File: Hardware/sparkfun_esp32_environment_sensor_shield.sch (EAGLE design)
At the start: 53 parts, among them J1 WEATHER_METER-WIND, J2 WEATHER_METER-RAIN, U1 BME280, U2 CCS811, U3 APDS-9301, U4 TVS Diode

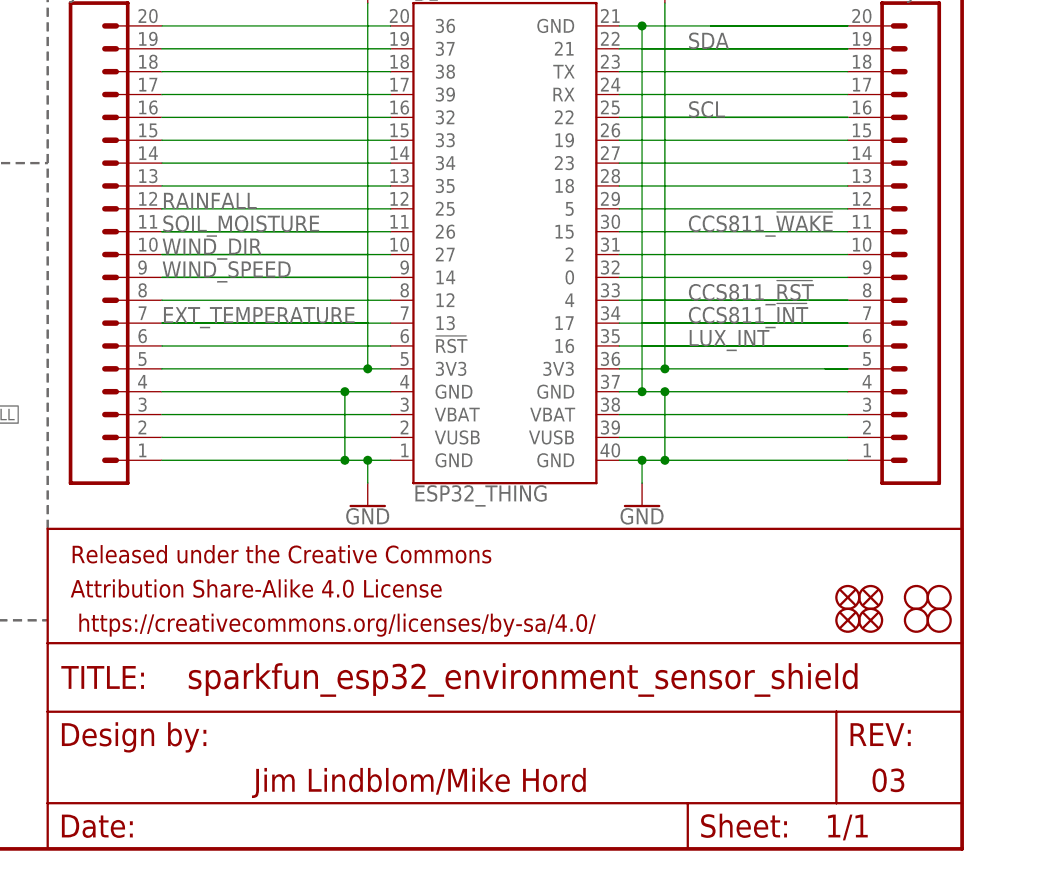
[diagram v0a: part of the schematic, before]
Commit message: Changes from review
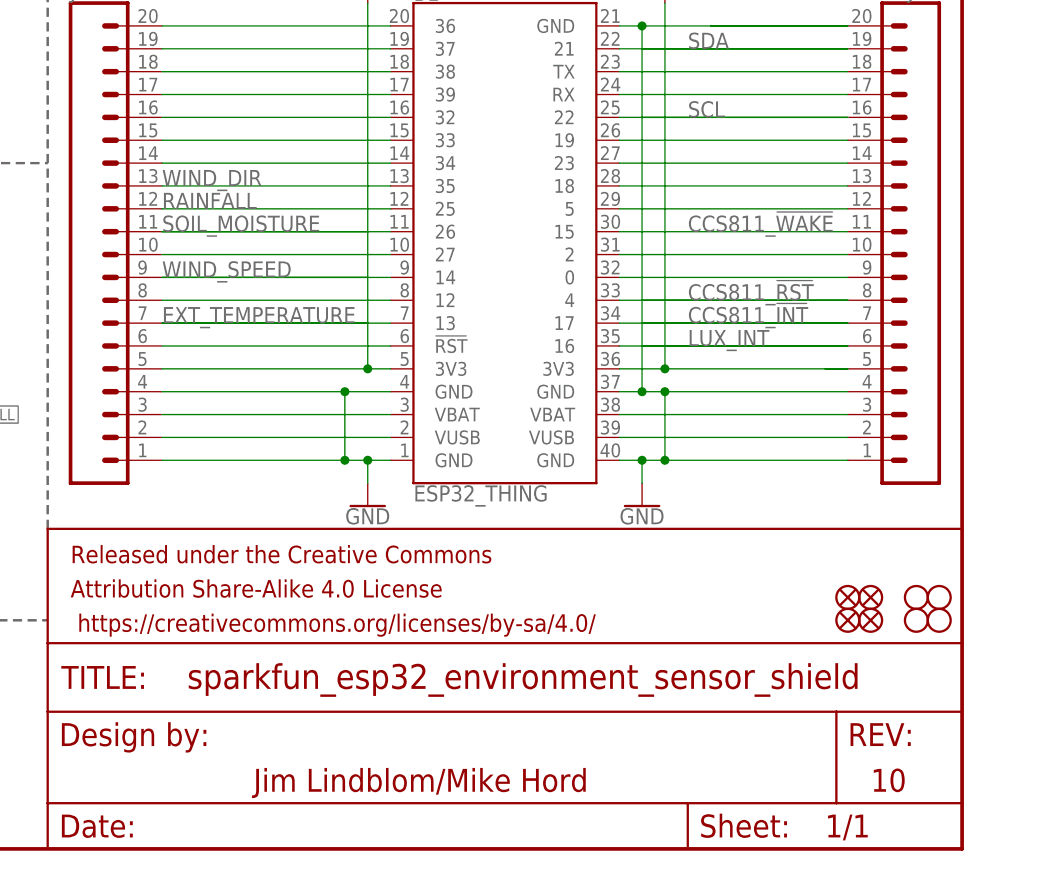
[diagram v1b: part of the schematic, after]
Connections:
- removed net N$10: B1.35, J4.13
- new net N$9: B1.27, J4.10
- net WIND_DIR: now also B1.35, J4.13; no longer B1.27, J4.10
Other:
- note added: "10"
- note removed: "03"
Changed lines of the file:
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@@
 to 4.7k pull-up
 resistors.</text>
-<text x="238.76" y="7.62" size="2.54" layer="94" align="center-left">03</text>
+<text x="238.76" y="7.62" size="2.54" layer="94" align="center-left">10</text>
 <text x="170.18" y="7.62" size="2.54" layer="94" align="center-left">Jim Lindblom/Mike Hord</text>
 <text x="119.38" y="20.32" size="1.27" layer="97" align="top-left">3-Pin temperature
@@
 </segment>
 <segment>
-<pinref part="B1" gate="G$1" pin="27"/>
-<wire x1="160.02" y1="66.04" x2="182.88" y2="66.04" width="0.1524" layer="91"/>
-<pinref part="J4" gate="G$1" pin="10"/>
-<wire x1="160.02" y1="66.04" x2="185.42" y2="66.04" width="0.1524" layer="91"/>
-<label x="160.02" y="66.04" size="1.778" layer="95"/>
-</segment>
-<segment>
 <wire x1="73.66" y1="58.42" x2="71.12" y2="58.42" width="0.1524" layer="91"/>
 <pinref part="U4" gate="U1" pin="IO4"/>
 <wire x1="73.66" y1="55.88" x2="73.66" y2="58.42" width="0.1524" layer="91"/>
 <label x="71.12" y="58.42" size="1.27" layer="95" rot="R180" xref="yes"/>
+</segment>
+<segment>
+<pinref part="B1" gate="G$1" pin="35"/>
+<pinref part="J4" gate="G$1" pin="13"/>
+<wire x1="160.02" y1="73.66" x2="185.42" y2="73.66" width="0.1524" layer="91"/>
+<label x="160.02" y="73.66" size="1.778" layer="95"/>
 </segment>
 </net>
@@
 </segment>
 </net>
-<net name="N$10" class="0">
-<segment>
-<pinref part="B1" gate="G$1" pin="35"/>
-<pinref part="J4" gate="G$1" pin="13"/>
-<wire x1="160.02" y1="73.66" x2="185.42" y2="73.66" width="0.1524" layer="91"/>
-</segment>
-</net>
 <net name="N$11" class="0">
 <segment>
@@
 </segment>
 </net>
+<net name="N$9" class="0">
+<segment>
+<pinref part="J4" gate="G$1" pin="10"/>
+<pinref part="B1" gate="G$1" pin="27"/>
+<wire x1="160.02" y1="66.04" x2="185.42" y2="66.04" width="0.1524" layer="91"/>
+</segment>
+</net>
